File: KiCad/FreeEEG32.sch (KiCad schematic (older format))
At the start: 45 parts, among them P11 CONN_01X03, SW1 NRST, SW2 BOOT0, U1 ADP7118AUJZ-3.3_TSOT, U12 MPU-6500, U2 ADP7118AUJZ-3.3_TSOT, U3 8.192MHz, U37 STM32F427ZI_4side_short, U39 ADP7118AUJZ-3.3_TSOT, U43 473521001, Y2 8MHz

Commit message: kicad
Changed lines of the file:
@@
 	4450 6400 4400 6400
 Wire Wire Line
-	4400 6400 4400 6350
+	4400 6350 4400 6400
 Wire Wire Line
-	4400 6350 4200 6350
+	4200 6350 4400 6350
 Wire Wire Line
 	4200 6350 4200 6400
@@
 	4450 6900 4400 6900
 Wire Wire Line
-	4400 6900 4400 6850
+	4400 6850 4400 6900
 Wire Wire Line
-	4400 6850 4200 6850
+	4200 6850 4400 6850
 Wire Wire Line
 	4200 6850 4200 6900
@@
 	4450 7400 4400 7400
 Wire Wire Line
-	4400 7400 4400 7350
+	4400 7350 4400 7400
 Wire Wire Line
-	4400 7350 4200 7350
+	4200 7350 4400 7350
 Wire Wire Line
 	4200 7350 4200 7400
@@
 	5900 6400 5850 6400
 Wire Wire Line
-	5850 6400 5850 6350
+	5850 6350 5850 6400
 Wire Wire Line
-	5850 6350 5650 6350
+	5650 6350 5850 6350
 Wire Wire Line
-	5650 6350 5650 6400
+	5650 6400 5650 6350
 Connection ~ 5750 6350
 Wire Wire Line
@@
 	5900 6900 5850 6900
 Wire Wire Line
-	5850 6900 5850 6850
+	5850 6850 5850 6900
 Wire Wire Line
-	5850 6850 5650 6850
+	5650 6850 5850 6850
 Wire Wire Line
-	5650 6850 5650 6900
+	5650 6900 5650 6850
 Connection ~ 5750 6850
 Wire Wire Line
@@
 	5900 7400 5850 7400
 Wire Wire Line
-	5850 7400 5850 7350
+	5850 7350 5850 7400
 Wire Wire Line
-	5850 7350 5650 7350
+	5650 7350 5850 7350
 Wire Wire Line
-	5650 7350 5650 7400
+	5650 7400 5650 7350
 Connection ~ 5750 7350
 Wire Wire Line
@@
 	4250 4550 4200 4550
 Wire Wire Line
-	4200 4550 4200 4600
+	4200 4600 4200 4550
 Connection ~ 4100 4600
 Wire Wire Line
@@
 	4200 4450 4250 4450
 Wire Wire Line
-	4200 4600 3900 4600
+	3900 4600 4200 4600
 Wire Wire Line
 	3900 4600 3900 4650

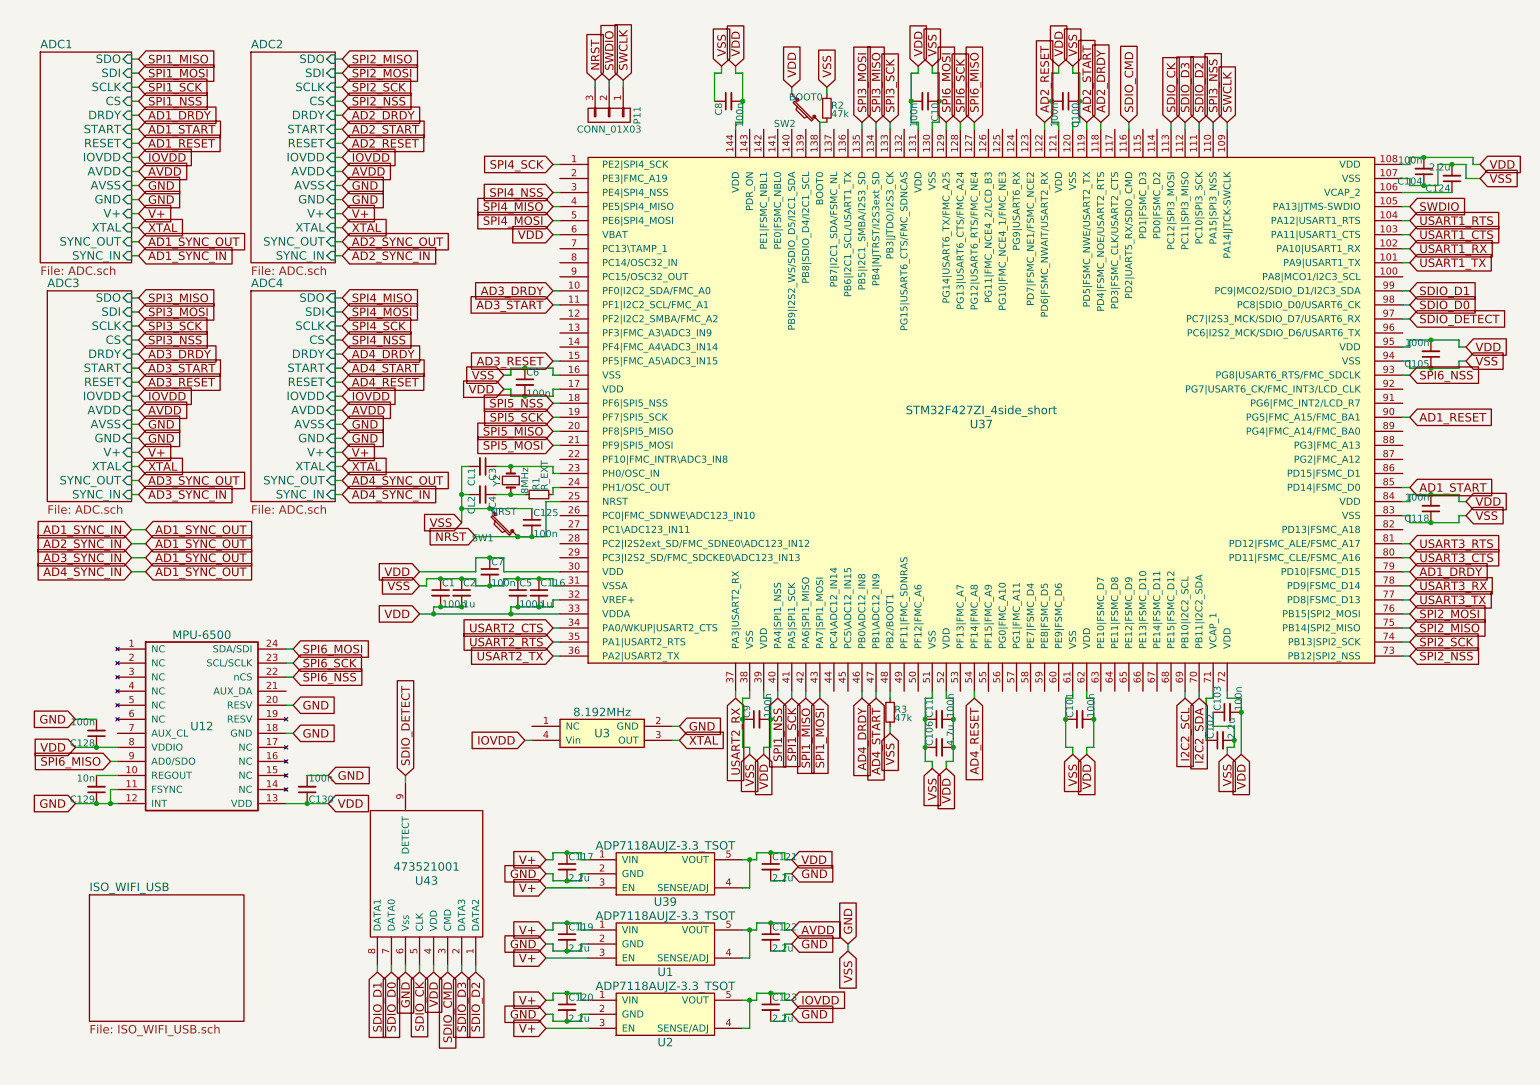
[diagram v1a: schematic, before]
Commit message: kicad
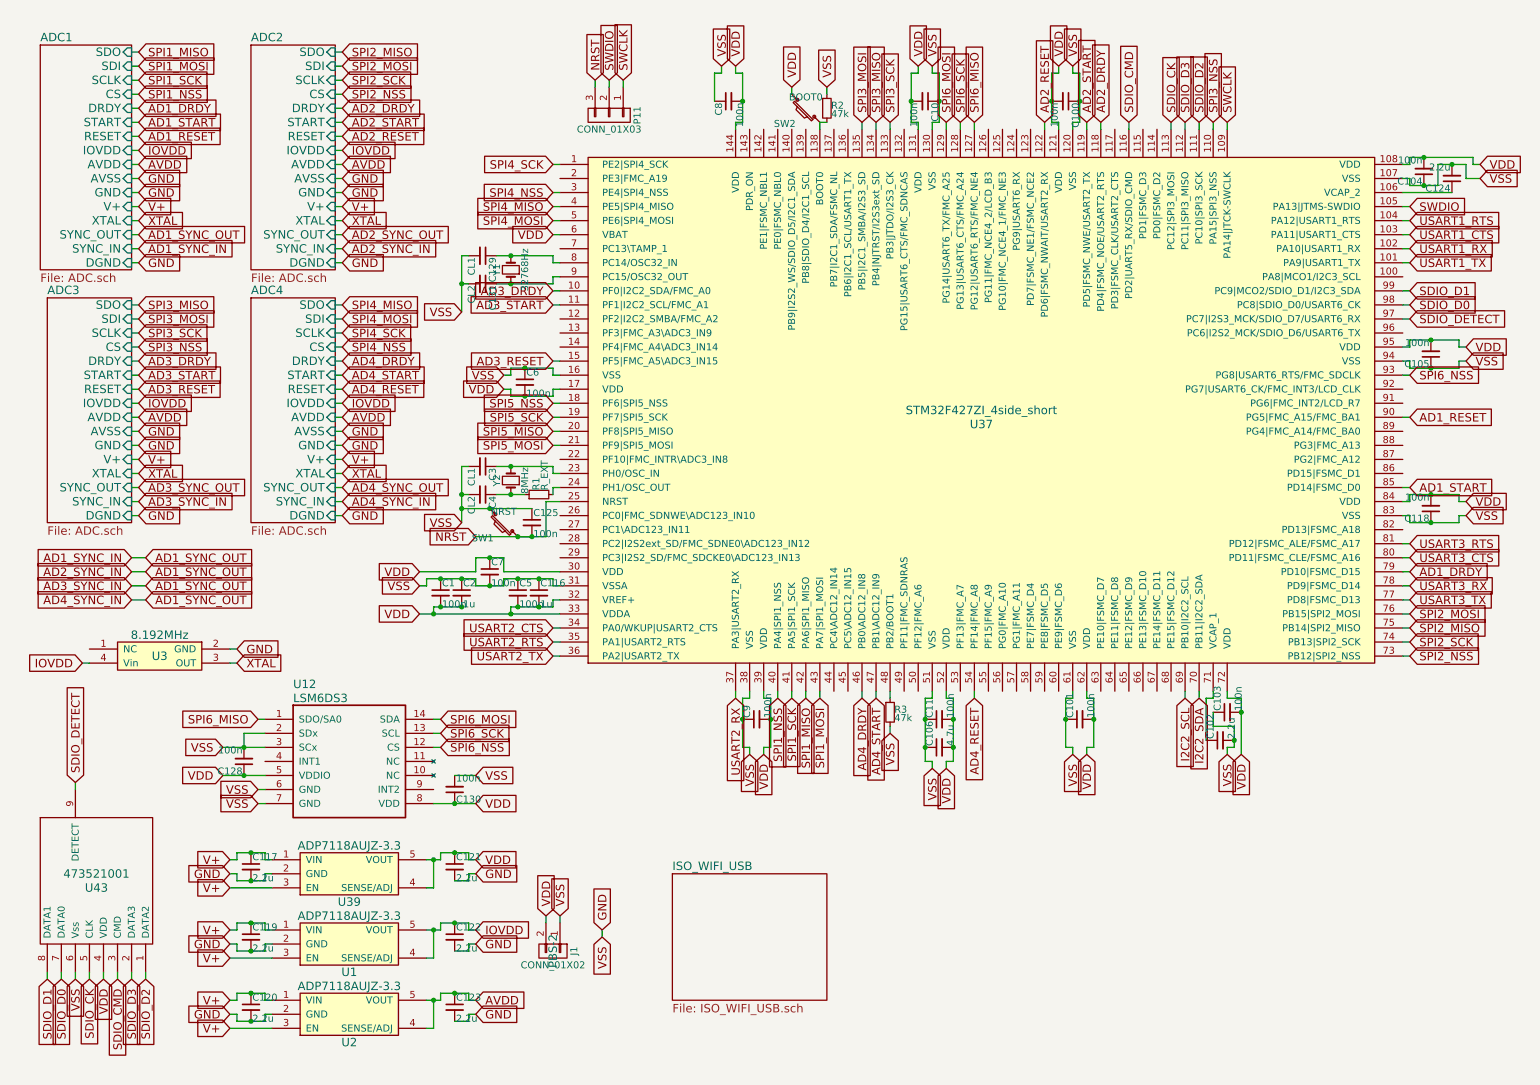
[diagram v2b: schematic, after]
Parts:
- removed U12: MPU-6500, Housings_DFN_QFN:QFN-24-1EP_4x4mm_Pitch0.5mm, symbol MPU-6500
- added C131: CL2, Capacitors_SMD:C_0402, symbol C_Small
- added J1: CONN_01X02, Socket_Strips:Socket_Strip_Straight_1x02, symbol CONN_01X02
- added U12: LSM6DS3, Housings_LGA_FreeEEG32:LGA-14L_2.5x3mm_Pitch0.5mm, symbol LSM6DS3
- added Y1: 32768Hz, Crystals:Crystal_SMD_MicroCrystal_CC4V-T1A-2pin_5.0x1.9mm, symbol Crystal_Small
- C129: value 10n -> CL1; manf# GRM155R71C103KA01D -> (none)
- SW1: manf# B3U3000PMB -> B3U-3000PM-B
- SW2: manf# B3U1000P -> B3U-1000P
- U1, U2, U39: value ADP7118AUJZ-3.3_TSOT -> ADP7118AUJZ-3.3
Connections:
- net AVDD: now also C123.1, U2.4 (SENSE/ADJ), U2.5 (VOUT); no longer C122.1, U1.4 (SENSE/ADJ), U1.5 (VOUT)
- net GND: now also C129.2, C131.2, J1.1 (P1), U12.2 (SDx), U12.3 (SCx), U12.6 (GND), U12.7 (GND); no longer C129.1
- net IOVDD: now also C122.1, U1.4 (SENSE/ADJ), U1.5 (VOUT); no longer C123.1, U2.4 (SENSE/ADJ), U2.5 (VOUT)
- net SPI6_MISO: now also U12.1 (SDO/SA0)
- net SPI6_MOSI: now also U12.14 (SDA)
- net SPI6_NSS: now also U12.12 (CS)
- net SPI6_SCK: now also U12.13 (SCL)
- net VDD: now also J1.2 (P2), U12.5 (VDDIO), U12.8 (VDD)
- net at U37.8 (PC14/OSC32_IN): now also C129.1, Y1.2
- net at U37.9 (PC15/OSC32_OUT): now also C131.1, Y1.1
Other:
- moved on the sheet: C117, C119, C120, C121, C122, C123, C128, C130, U1, U2, U3, U39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
